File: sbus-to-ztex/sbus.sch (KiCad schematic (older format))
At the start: 24 parts, among them U1 SN74CB3T16211DGGR, U10 74CB3T1G125, U2 SN74CB3T16211DGGR, U3 SN74CB3T16211DGGR, U4 74CB3T1G125

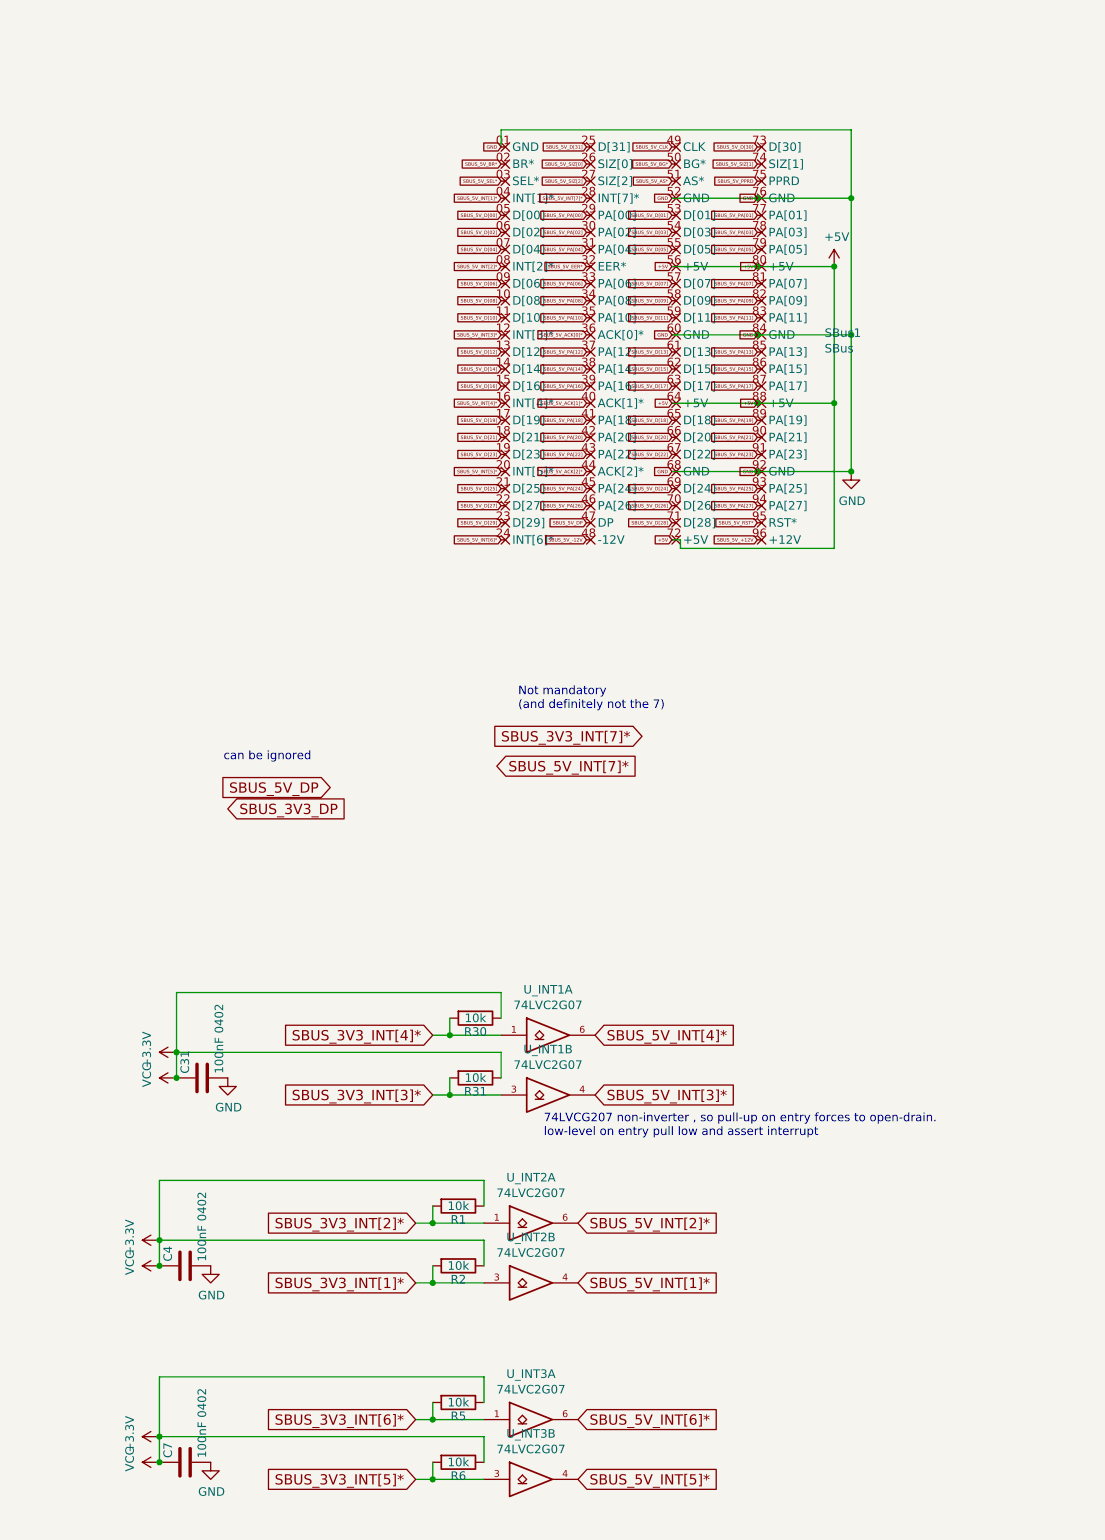
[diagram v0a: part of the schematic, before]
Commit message: more V1.3
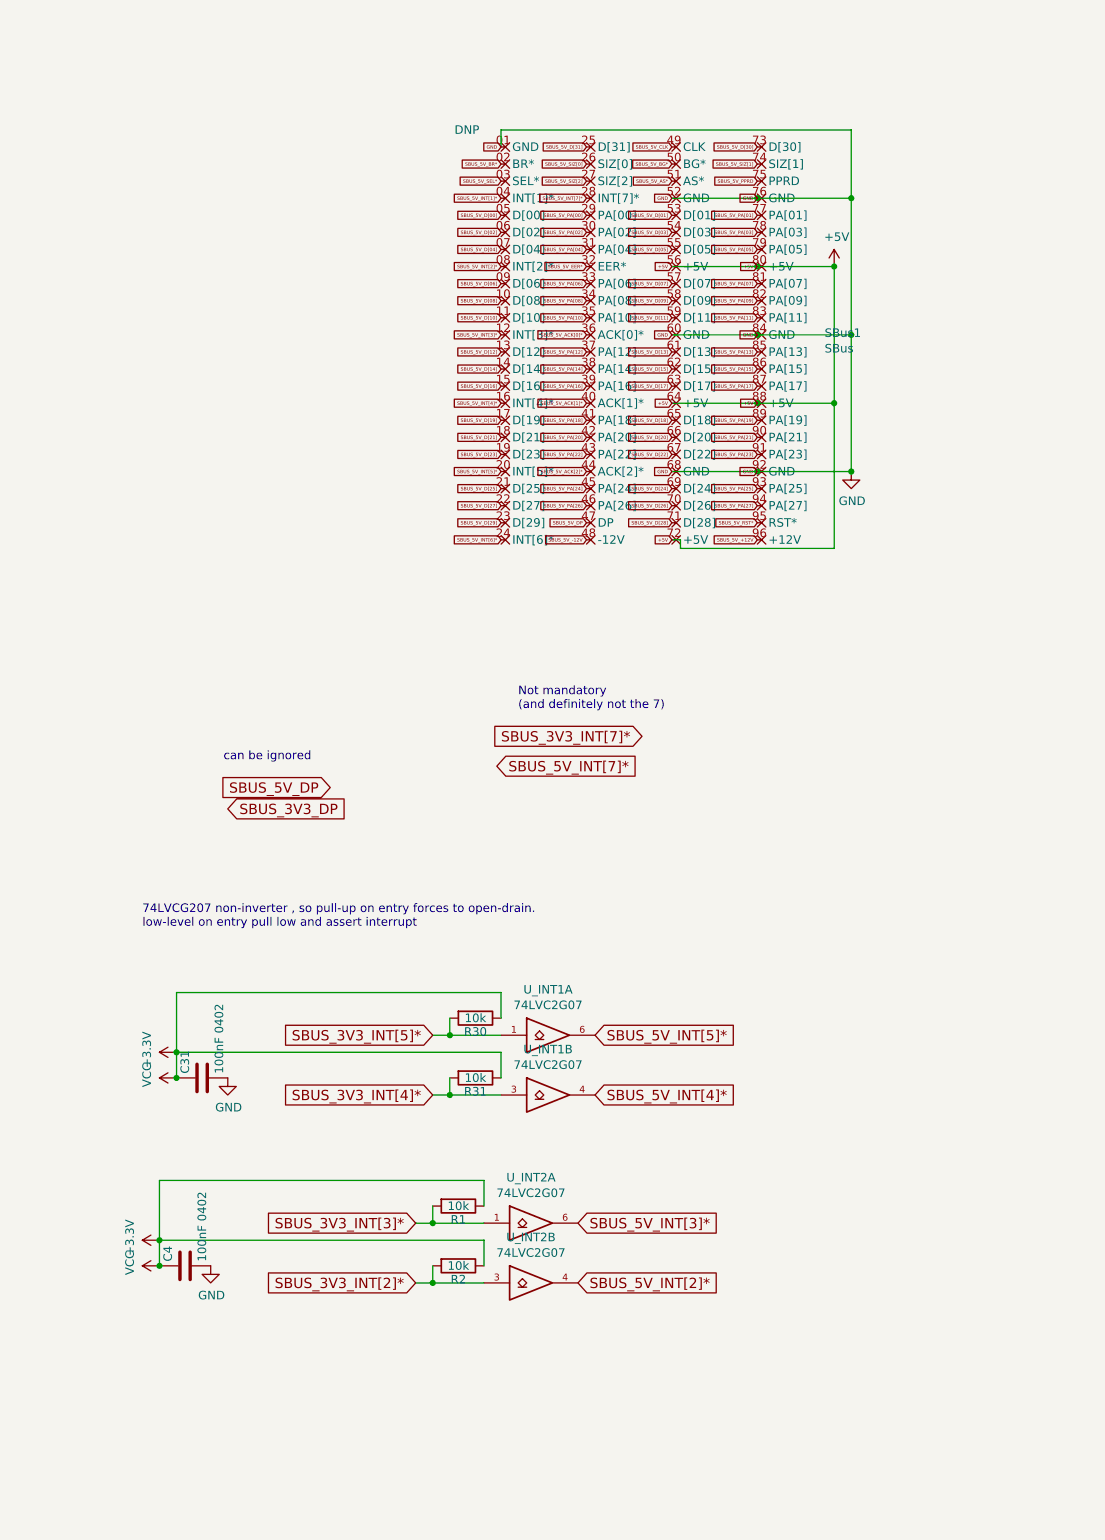
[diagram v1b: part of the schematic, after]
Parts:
- removed C7: 100nF 0402, Capacitor_SMD:C_0402_1005Metric, symbol Device:C
- removed R5, R6: 10k, Resistor_SMD:R_0402_1005Metric, symbol Device:R
- removed U_INT3: 74LVC2G07, For_SeeedStudio:SOT65P210X110-6N, symbol 74xGxx:74AUC2G07
- SBus1: DNP (none) -> DNP
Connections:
- net SBUS_3V3_INT[1]* is gone; now on net SBUS_3V3_INT[2]*: R2.2, U_INT2.3
- net SBUS_3V3_INT[2]*: no longer R1.2, U_INT2.1
- net SBUS_3V3_INT[3]*: now also R1.2, U_INT2.1; no longer R31.2, U_INT1.3
- net SBUS_3V3_INT[4]*: now also R31.2, U_INT1.3; no longer R30.2, U_INT1.1
- net SBUS_3V3_INT[5]*: now also R30.2, U_INT1.1
- net SBUS_5V_INT[1]*: no longer U_INT2.4
- net SBUS_5V_INT[2]*: now also U_INT2.4; no longer U_INT2.6
- net SBUS_5V_INT[3]*: now also U_INT2.6; no longer U_INT1.4
- net SBUS_5V_INT[4]*: now also U_INT1.4; no longer U_INT1.6
- net SBUS_5V_INT[5]*: now also U_INT1.6
